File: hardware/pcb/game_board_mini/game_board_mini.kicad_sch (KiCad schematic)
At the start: 8 parts, among them J1 Conn_01x08, J2 Conn_01x03_Male, J3 Conn_01x03, J4 Conn_01x03, J5 Conn_01x03

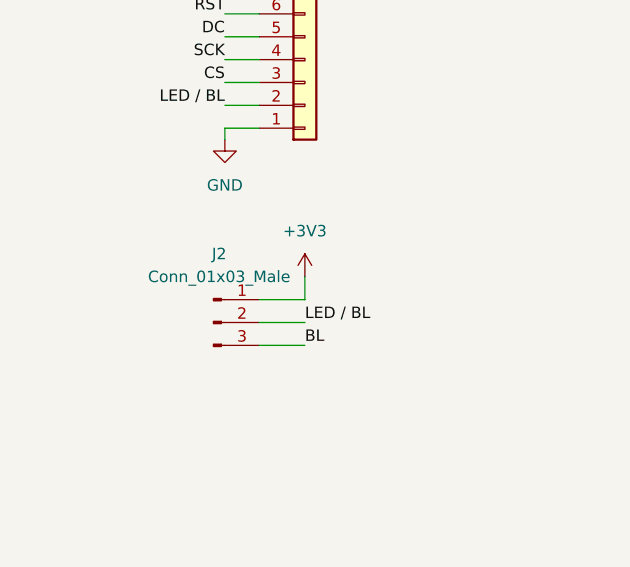
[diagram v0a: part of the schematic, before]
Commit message: [PCB] Routed ESP
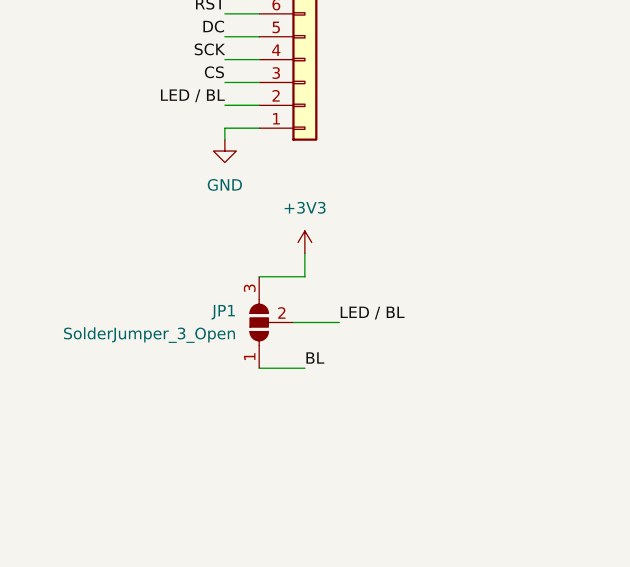
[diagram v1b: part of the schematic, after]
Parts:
- removed J2: Conn_01x03_Male, Connector_PinHeader_2.54mm:PinHeader_1x03_P2.54mm_Vertical, symbol Connector:Conn_01x03_Male
- added JP1: SolderJumper_3_Open, Jumper:SolderJumper-3_P1.3mm_Open_Pad1.0x1.5mm, symbol Jumper:SolderJumper_3_Open
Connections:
- net +3V3: now also JP1.3 (B)
- net BL: now also JP1.1 (A)
- net LED / BL: now also JP1.2 (C)
